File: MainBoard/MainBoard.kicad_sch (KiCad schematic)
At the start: 23 parts, among them J1 1761681-3, U1 TL072CP

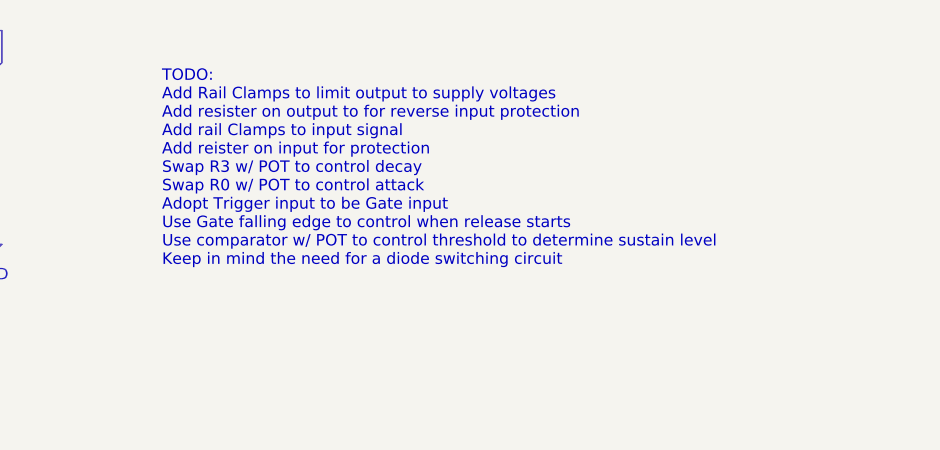
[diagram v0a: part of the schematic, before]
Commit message: updated notes
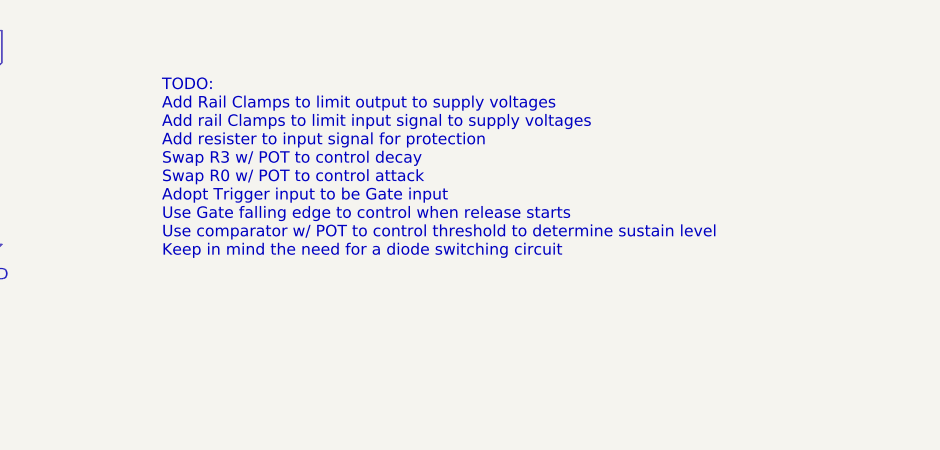
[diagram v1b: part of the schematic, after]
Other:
- note added: "TODO: Add Rail Clamps to limit output to supply voltages Add rail Clamps to limit input signal to supply voltages Add resister to input signal for protection Swap R3 w/ POT to control decay Swap R0 w/ POT to control attack Adopt Trigger input to be Gate input Use Gate falling edge to control when release starts Use comparator w/ POT to control threshold to determine sustain level Keep in mind the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"
- note removed: "TODO: Add Rail Clamps to limit output to supply voltages Add resister on output to for reverse input protection Add rail Clamps to input signal Add reister on input for protection Swap R3 w/ POT to control decay Swap R0 w/ POT to control attack Adopt Trigger input to be Gate input Use Gate falling edge to control when release starts Use comparator w/ POT to control threshold to determine sustain 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"
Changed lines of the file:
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@@
 		(company "R-mods")
 	)
-	(text "TODO:\nAdd Rail Clamps to limit output to supply voltages\nAdd resister on output to for reverse input protection\nAdd rail Clamps to input signal\nAdd reister on input for protection\nSwap R3 w/ POT to control decay\nSwap R0 w/ POT to control attack\nAdopt Trigger input to be Gate input\nUse Gate falling edge to control when release starts\nUse comparator w/ POT to control threshold to determine sustain level\nKeep in mind the need for a diode switching circuit\n\n"
+	(text "TODO:\nAdd Rail Clamps to limit output to supply voltages\nAdd rail Clamps to limit input signal to supply voltages\nAdd resister to input signal for protection\nSwap R3 w/ POT to control decay\nSwap R0 w/ POT to control attack\nAdopt Trigger input to be Gate input\nUse Gate falling edge to control when release starts\nUse comparator w/ POT to control threshold to determine sustain level\nKeep in mind the need for a diode switching circuit\n\n"
 		(exclude_from_sim no)
 		(at 203.2 47.244 0)
